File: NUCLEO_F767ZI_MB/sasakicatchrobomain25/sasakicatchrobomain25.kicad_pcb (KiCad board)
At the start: 2 copper layers, 116 x 93.9 mm, 31 parts, among them J3 XT60-M, J4 Conn_02x08_Odd_Even, J6 Conn_02x10_Odd_Even, J7 Conn_02x17_Odd_Even, J8 Conn_02x15_Odd_Even

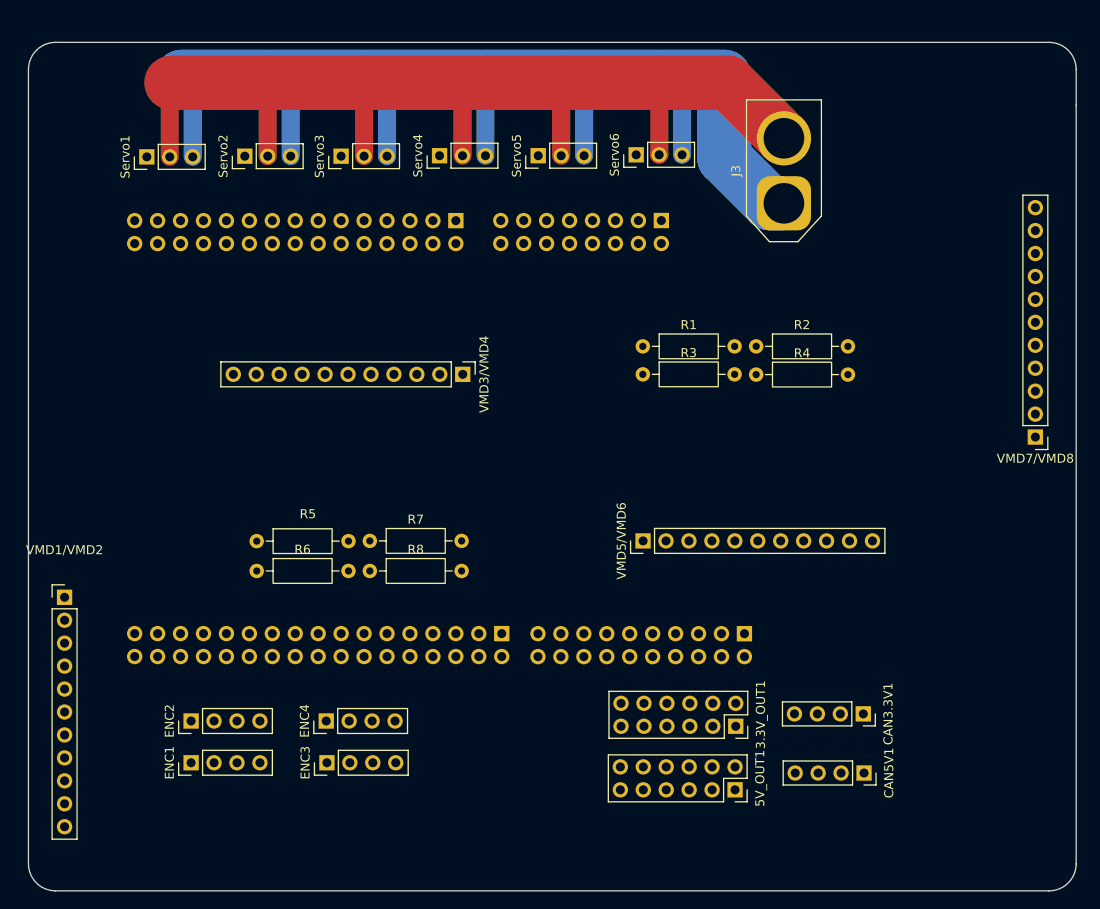
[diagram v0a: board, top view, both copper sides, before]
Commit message: 基盤購入しました!!!!
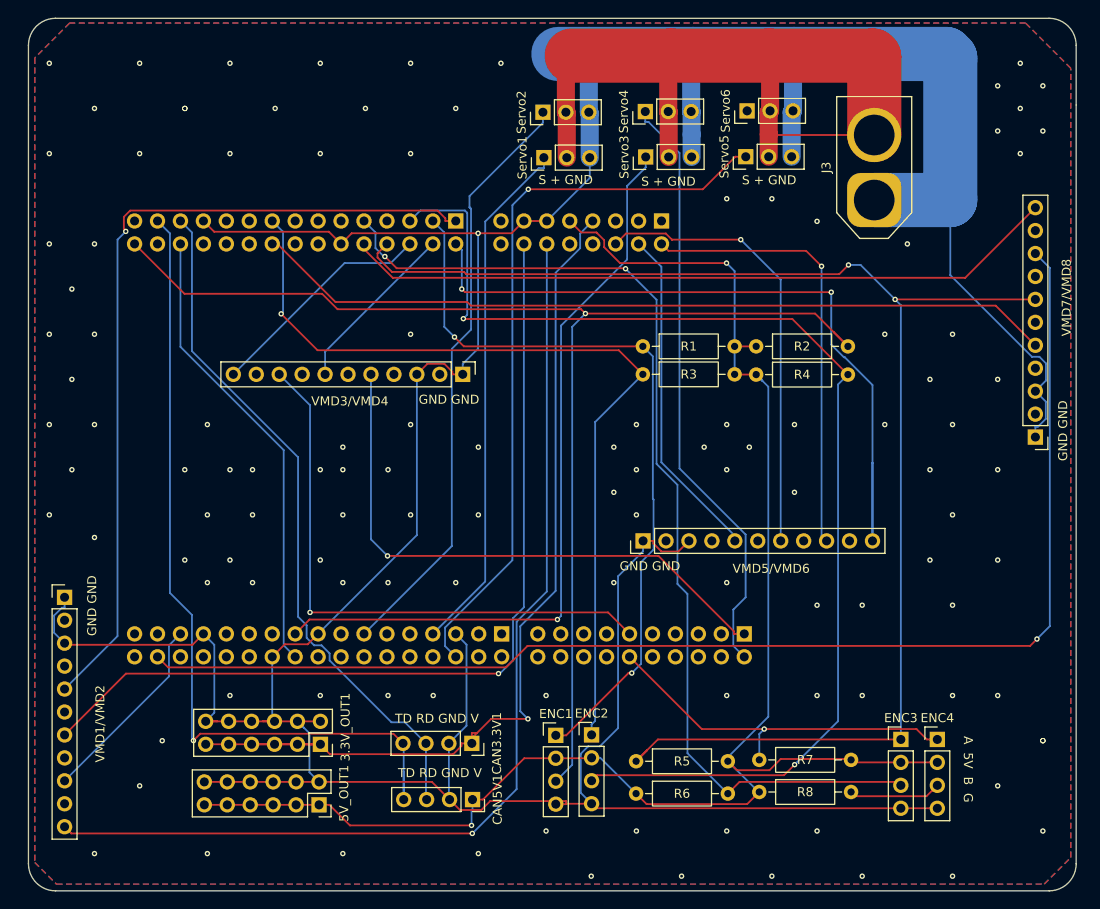
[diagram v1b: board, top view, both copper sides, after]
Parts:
- moved ENC4 67.7 mm to (168.9, 124.0), turned to 0 degrees
- moved ENC3 63.6 mm to (164.8, 124.0), turned to 0 degrees
- moved R8 49.6 mm to (149.2, 129.8)
- moved R7 49.5 mm to (149.2, 126.2)
- moved R6 48.7 mm to (135.5, 130.0)
- moved R5 48.6 mm to (135.5, 126.4)
- moved 5V_OUT1 46.1 mm to (100.4, 131.2)
- moved 3.3V_OUT1 46.0 mm to (100.6, 124.5)
- moved ENC2 44.4 mm to (130.6, 123.5), turned to 0 degrees
- moved Servo1 44.0 mm to (125.3, 59.6)
- moved CAN3.3V1 43.5 mm to (117.3, 124.4)
- moved CAN5V1 43.4 mm to (117.4, 130.6)
- moved ENC1 40.5 mm to (126.6, 123.5), turned to 0 degrees
- moved Servo3 33.7 mm to (136.6, 59.5)
- moved Servo2 33.4 mm to (125.2, 54.5)
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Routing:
- net GND: track 131.2 -> 458.7 mm, vias 0 -> 120
- net +5V: track 0.00 -> 183.5 mm, vias 0 -> 2
- net PD_4: track 0.00 -> 158.5 mm, vias 0 -> 2
- net PB_10: track 0.00 -> 143.1 mm, vias 0 -> 1
- net PG_1: track 0.00 -> 139.0 mm, vias 0 -> 1
- net PC_3: track 0.00 -> 132.9 mm, vias 0 -> 2
- net PF_5: track 0.00 -> 114.8 mm, vias 0 -> 2
- net PD_2: track 0.00 -> 114.1 mm, vias 0 -> 1
- net +3.3V: track 0.00 -> 110.5 mm, vias 0 -> 1
- net PG_2: track 0.00 -> 99.7 mm, vias 0 -> 1
- net PF_2: track 0.00 -> 96.0 mm, vias 0 -> 1
- net PD_1: track 0.00 -> 93.2 mm, vias 0 -> 1
- net PA_3: track 0.00 -> 92.9 mm, vias 0 -> 1
- net PE_5: track 0.00 -> 89.1 mm
- net PD_13: track 0.00 -> 85.5 mm, vias 0 -> 1
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- added copper zone on B.Cu, net GND
- added copper zone on F.Cu, net GND
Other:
- board size 116 x 93.9 mm -> 116 x 96.6 mm
- board text added: "A 5V B G"
- board text added: "GND GND"
- board text added: "S + GND"
- board text added: "TD RD GND V"
